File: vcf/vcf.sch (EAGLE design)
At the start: 94 parts, among them IC1 OPA4130U, IC2 OPA4130U, IC3 OPA4130U, IC4 OPA4130U, IC5 OPA4130U, Q1 BC847ASMD, Q2 BC847ASMD, Q3 BC847ASMD, Q4 BC847ASMD, Q5 BC847ASMD, Q6 BC847ASMD

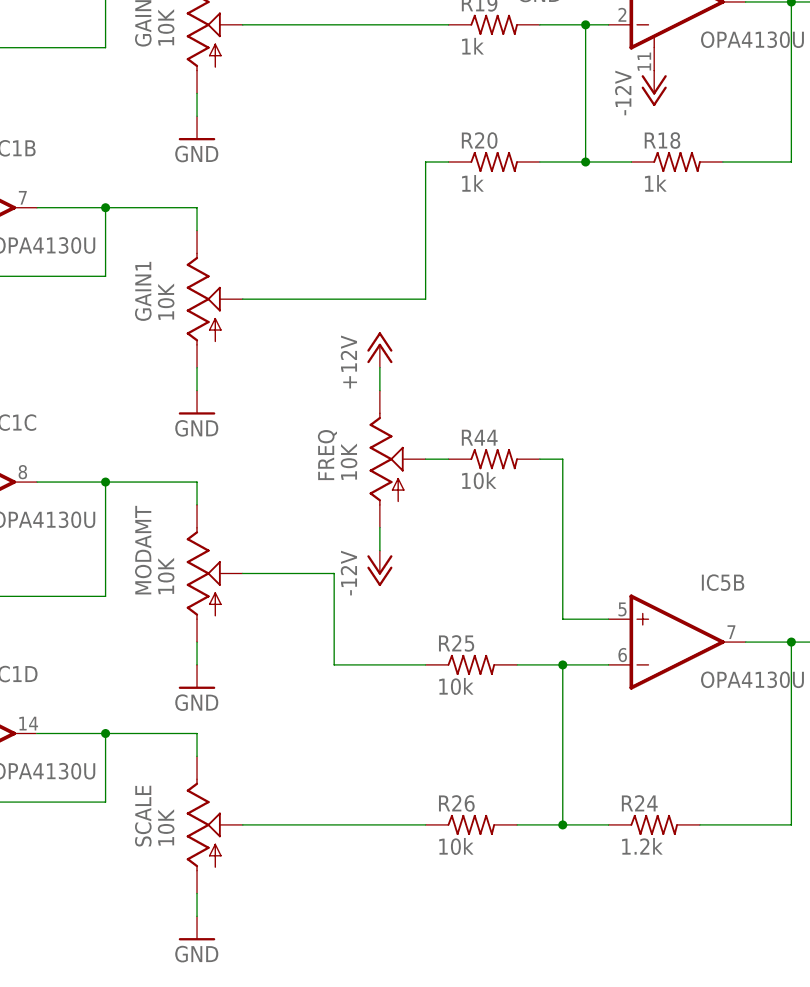
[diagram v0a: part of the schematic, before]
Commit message: added some critical stuff.  sent the board to pcbway for checking.
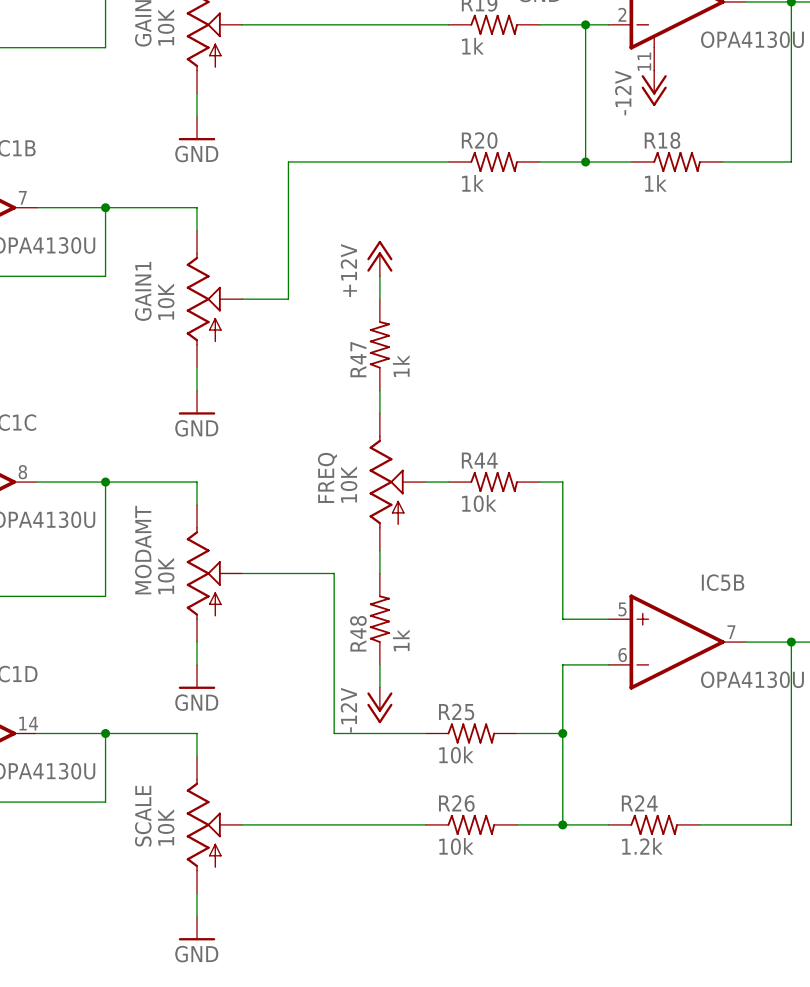
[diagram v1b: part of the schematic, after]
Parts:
- added R47, R48: 1k, dan:R-US_R0603
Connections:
- new net N$65: FREQ.A, R48.2
- new net N$66: FREQ.E, R47.1
- net +12V: now also R47.2; no longer FREQ.E
- net -12V: now also R48.1; no longer FREQ.A
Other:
- moved on the sheet: FREQ, R25, R44
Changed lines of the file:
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@@
 <part name="R45" library="dan" deviceset="R-US_" device="R0603" value="1k"/>
 <part name="R46" library="dan" deviceset="R-US_" device="R0603" value="1k"/>
+<part name="R47" library="dan" deviceset="R-US_" device="R0603" value="1k"/>
+<part name="R48" library="dan" deviceset="R-US_" device="R0603" value="1k"/>
 </parts>
 <sheets>
@@
 <instance part="R23" gate="G$1" x="-20.32" y="-33.02"/>
 <instance part="R24" gate="G$1" x="-48.26" y="-53.34"/>
-<instance part="R25" gate="G$1" x="-68.58" y="-35.56"/>
+<instance part="R25" gate="G$1" x="-68.58" y="-43.18"/>
 <instance part="R26" gate="G$1" x="-68.58" y="-53.34"/>
 <instance part="MODAMT" gate="G$1" x="-99.06" y="-25.4"/>
@@
 <instance part="GND20" gate="1" x="208.28" y="73.66"/>
 <instance part="GND21" gate="1" x="149.86" y="200.66"/>
-<instance part="FREQ" gate="G$1" x="-78.74" y="-12.7"/>
-<instance part="P-7" gate="1" x="-78.74" y="-25.4"/>
-<instance part="P+9" gate="1" x="-78.74" y="0"/>
-<instance part="R44" gate="G$1" x="-66.04" y="-12.7"/>
+<instance part="FREQ" gate="G$1" x="-78.74" y="-15.24"/>
+<instance part="P-7" gate="1" x="-78.74" y="-40.64"/>
+<instance part="P+9" gate="1" x="-78.74" y="10.16"/>
+<instance part="R44" gate="G$1" x="-66.04" y="-15.24"/>
 <instance part="GAIN1" gate="G$1" x="-99.06" y="5.08"/>
 <instance part="C5" gate="G$1" x="-2.54" y="38.1" rot="R270"/>
@@
 <instance part="R45" gate="G$1" x="205.74" y="66.04" rot="R180"/>
 <instance part="R46" gate="G$1" x="147.32" y="193.04" rot="R180"/>
+<instance part="R47" gate="G$1" x="-78.74" y="0" rot="R90"/>
+<instance part="R48" gate="G$1" x="-78.74" y="-30.48" rot="R90"/>
 </instances>
 <busses>
@@
 </segment>
 <segment>
-<pinref part="FREQ" gate="G$1" pin="E"/>
-<pinref part="P+9" gate="1" pin="+12V"/>
-<wire x1="-78.74" y1="-5.08" x2="-78.74" y2="-2.54" width="0.1524" layer="91"/>
-</segment>
-<segment>
 <pinref part="P+10" gate="1" pin="+12V"/>
 <wire x1="-12.7" y1="154.94" x2="-12.7" y2="152.4" width="0.1524" layer="91"/>
@@
 <pinref part="P+7" gate="1" pin="+12V"/>
 </segment>
+<segment>
+<pinref part="R47" gate="G$1" pin="2"/>
+<pinref part="P+9" gate="1" pin="+12V"/>
+<wire x1="-78.74" y1="7.62" x2="-78.74" y2="5.08" width="0.1524" layer="91"/>
+</segment>
 </net>
 <net name="-12V" class="0">
@@
 <wire x1="-50.8" y1="177.8" x2="-40.64" y2="177.8" width="0.1524" layer="91"/>
 <junction x="-50.8" y="177.8"/>
-</segment>
-<segment>
-<pinref part="P-7" gate="1" pin="-12V"/>
-<pinref part="FREQ" gate="G$1" pin="A"/>
-<wire x1="-78.74" y1="-22.86" x2="-78.74" y2="-20.32" width="0.1524" layer="91"/>
 </segment>
 <segment>
@@
 <pinref part="P-5" gate="1" pin="-12V"/>
 </segment>
+<segment>
+<pinref part="P-7" gate="1" pin="-12V"/>
+<pinref part="R48" gate="G$1" pin="1"/>
+<wire x1="-78.74" y1="-38.1" x2="-78.74" y2="-35.56" width="0.1524" layer="91"/>
+</segment>
 </net>
 <net name="N$17" class="0">
@@
 <wire x1="-63.5" y1="-53.34" x2="-58.42" y2="-53.34" width="0.1524" layer="91"/>
 <junction x="-58.42" y="-53.34"/>
-<wire x1="-58.42" y1="-35.56" x2="-58.42" y2="-53.34" width="0.1524" layer="91"/>
+<wire x1="-58.42" y1="-35.56" x2="-58.42" y2="-43.18" width="0.1524" layer="91"/>
+<wire x1="-58.42" y1="-43.18" x2="-58.42" y2="-53.34" width="0.1524" layer="91"/>
+<wire x1="-53.34" y1="-35.56" x2="-58.42" y2="-35.56" width="0.1524" layer="91"/>
+<pinref part="IC5" gate="B" pin="-IN"/>
 <pinref part="R25" gate="G$1" pin="2"/>
-<wire x1="-63.5" y1="-35.56" x2="-58.42" y2="-35.56" width="0.1524" layer="91"/>
-<wire x1="-53.34" y1="-35.56" x2="-58.42" y2="-35.56" width="0.1524" layer="91"/>
-<junction x="-58.42" y="-35.56"/>
-<pinref part="IC5" gate="B" pin="-IN"/>
+<wire x1="-63.5" y1="-43.18" x2="-58.42" y2="-43.18" width="0.1524" layer="91"/>
+<junction x="-58.42" y="-43.18"/>
 </segment>
 </net>
@@
 <net name="N$40" class="0">
 <segment>
-<pinref part="R25" gate="G$1" pin="1"/>
-<wire x1="-73.66" y1="-35.56" x2="-83.82" y2="-35.56" width="0.1524" layer="91"/>
-<wire x1="-83.82" y1="-35.56" x2="-83.82" y2="-25.4" width="0.1524" layer="91"/>
+<wire x1="-83.82" y1="-43.18" x2="-83.82" y2="-25.4" width="0.1524" layer="91"/>
 <pinref part="MODAMT" gate="G$1" pin="S"/>
 <wire x1="-83.82" y1="-25.4" x2="-93.98" y2="-25.4" width="0.1524" layer="91"/>
+<pinref part="R25" gate="G$1" pin="1"/>
+<wire x1="-73.66" y1="-43.18" x2="-83.82" y2="-43.18" width="0.1524" layer="91"/>
 </segment>
 </net>
@@
 <pinref part="FREQ" gate="G$1" pin="S"/>
 <pinref part="R44" gate="G$1" pin="1"/>
-<wire x1="-73.66" y1="-12.7" x2="-71.12" y2="-12.7" width="0.1524" layer="91"/>
+<wire x1="-73.66" y1="-15.24" x2="-71.12" y2="-15.24" width="0.1524" layer="91"/>
 </segment>
 </net>
 <net name="N$62" class="0">
 <segment>
-<wire x1="-73.66" y1="5.08" x2="-73.66" y2="20.32" width="0.1524" layer="91"/>
+<wire x1="-88.9" y1="5.08" x2="-88.9" y2="20.32" width="0.1524" layer="91"/>
 <pinref part="R20" gate="G$1" pin="1"/>
-<wire x1="-73.66" y1="20.32" x2="-71.12" y2="20.32" width="0.1524" layer="91"/>
+<wire x1="-88.9" y1="20.32" x2="-71.12" y2="20.32" width="0.1524" layer="91"/>
 <pinref part="GAIN1" gate="G$1" pin="S"/>
-<wire x1="-93.98" y1="5.08" x2="-73.66" y2="5.08" width="0.1524" layer="91"/>
+<wire x1="-93.98" y1="5.08" x2="-88.9" y2="5.08" width="0.1524" layer="91"/>
 </segment>
 </net>
@@
 <pinref part="IC5" gate="B" pin="+IN"/>
 <pinref part="R44" gate="G$1" pin="2"/>
-<wire x1="-58.42" y1="-12.7" x2="-60.96" y2="-12.7" width="0.1524" layer="91"/>
-<wire x1="-58.42" y1="-30.48" x2="-58.42" y2="-12.7" width="0.1524" layer="91"/>
+<wire x1="-58.42" y1="-15.24" x2="-60.96" y2="-15.24" width="0.1524" layer="91"/>
+<wire x1="-58.42" y1="-30.48" x2="-58.42" y2="-15.24" width="0.1524" layer="91"/>
 </segment>
 </net>
@@
 </segment>
 </net>
+<net name="N$65" class="0">
+<segment>
+<pinref part="FREQ" gate="G$1" pin="A"/>
+<pinref part="R48" gate="G$1" pin="2"/>
+<wire x1="-78.74" y1="-25.4" x2="-78.74" y2="-22.86" width="0.1524" layer="91"/>
+</segment>
+</net>
+<net name="N$66" class="0">
+<segment>
+<pinref part="FREQ" gate="G$1" pin="E"/>
+<pinref part="R47" gate="G$1" pin="1"/>
+<wire x1="-78.74" y1="-5.08" x2="-78.74" y2="-7.62" width="0.1524" layer="91"/>
+</segment>
+</net>
